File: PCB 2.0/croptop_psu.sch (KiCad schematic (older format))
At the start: 35 parts, among them J3 5V USB, U2 REG71055, U3 FAN5333BSX, U4 MIC23050, U5 TC1014

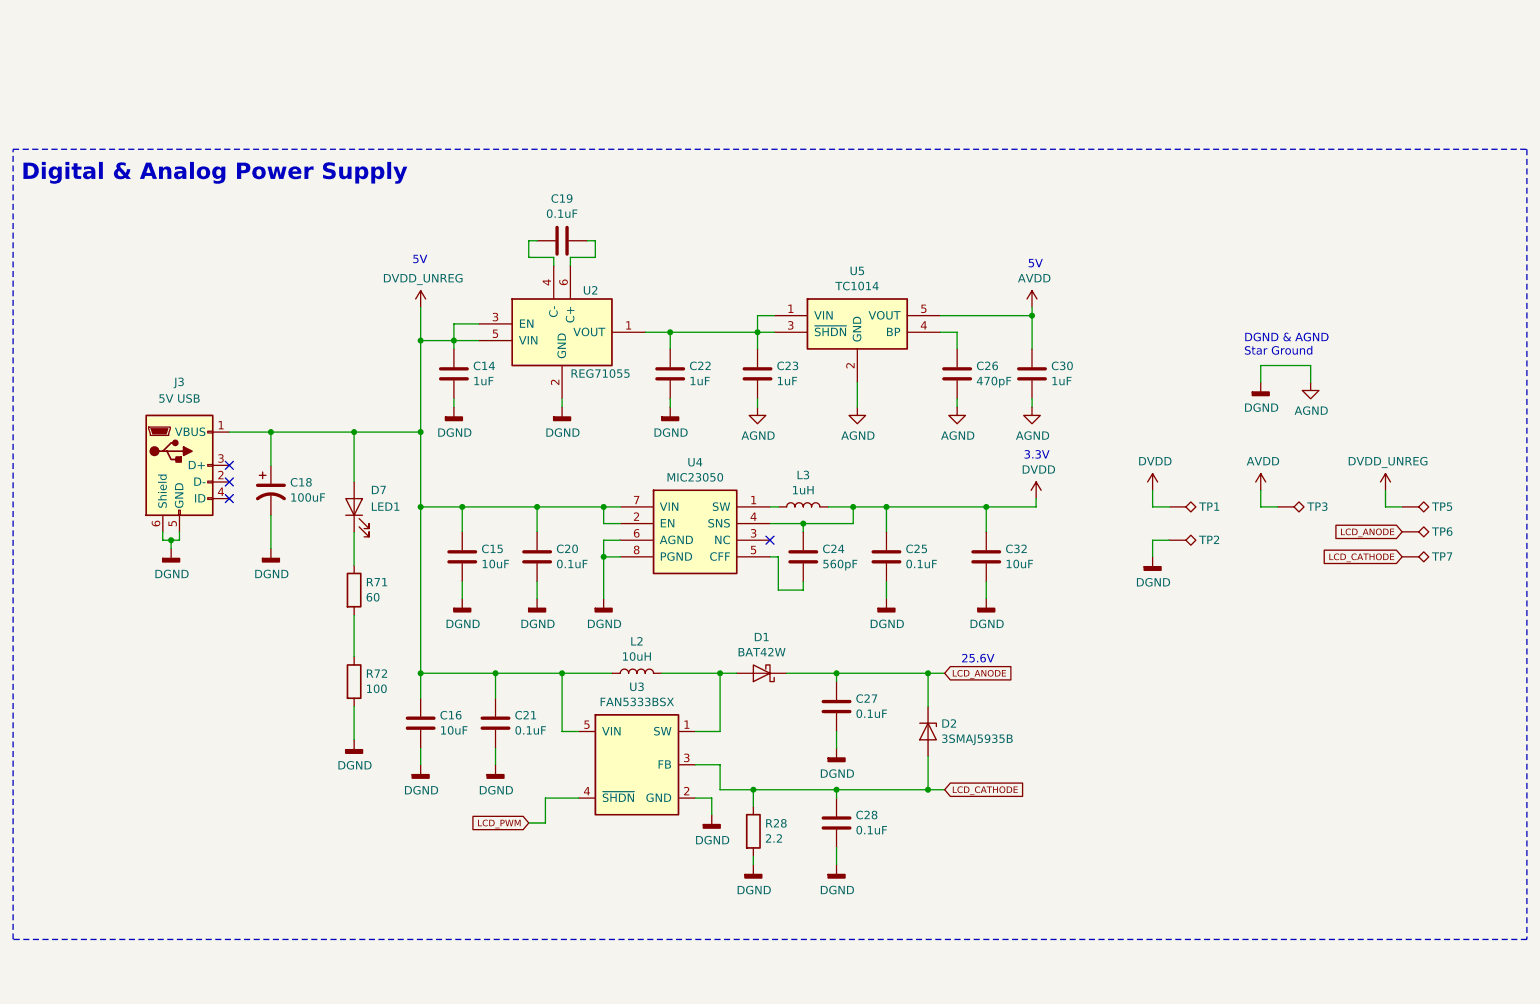
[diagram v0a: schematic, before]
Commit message: Fixed it
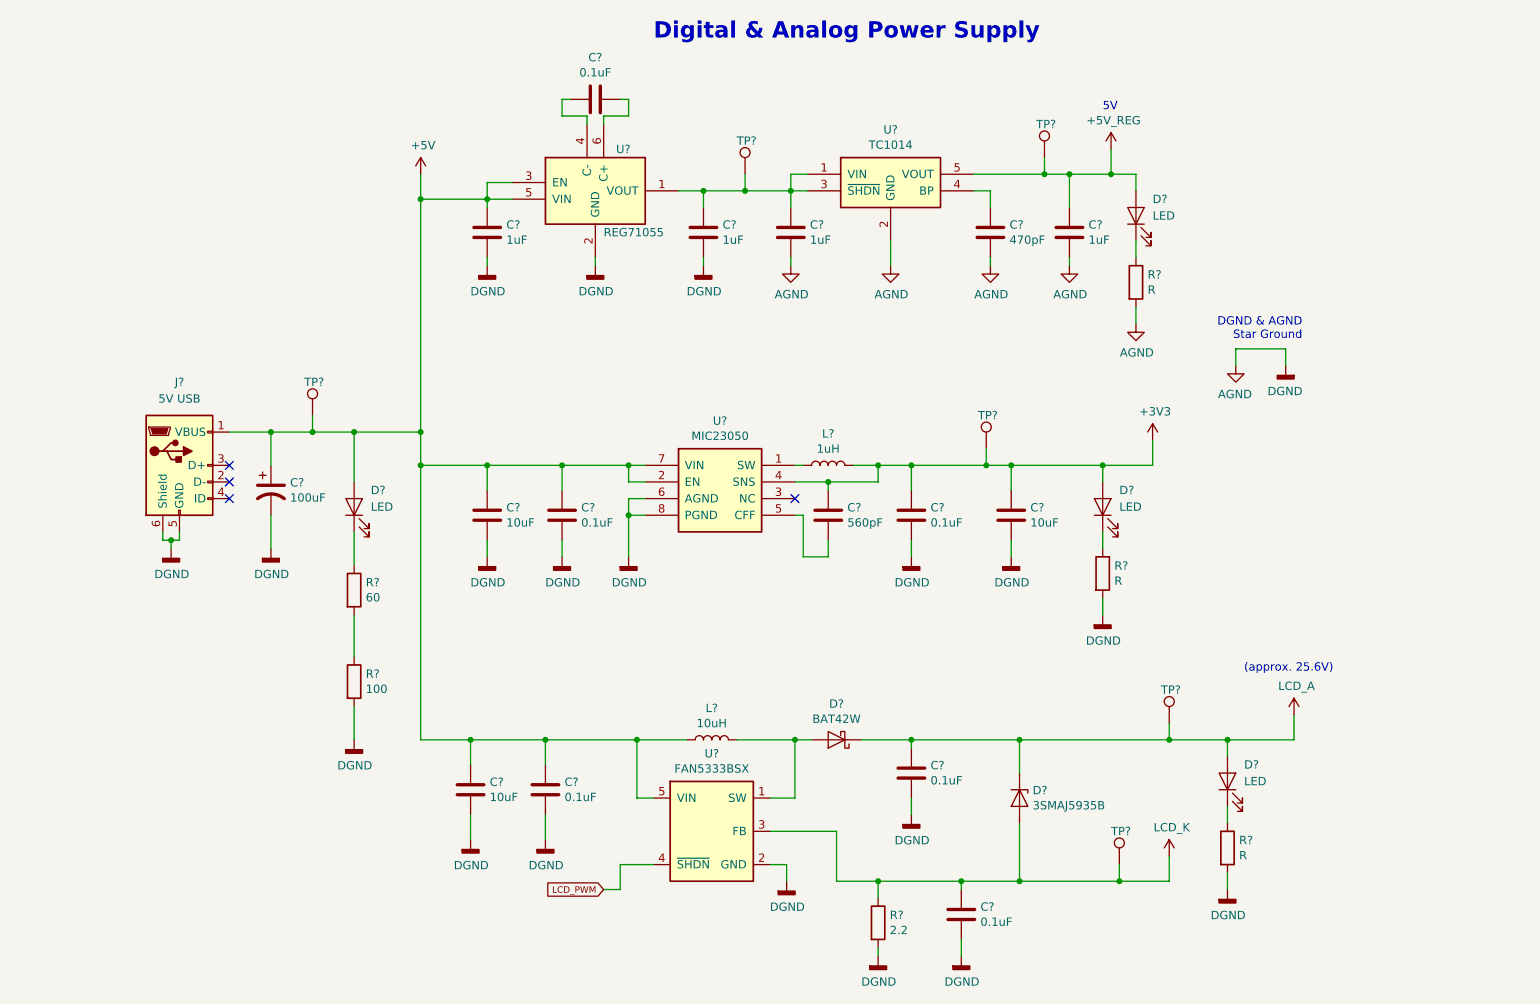
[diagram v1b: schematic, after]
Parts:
- removed TP1, TP2, TP3, TP5, TP6, TP7: TestPoint_Alt, croptop:TestPoint, symbol Connector:TestPoint_Alt
- added D? (x3): LED, LED_SMD:LED_0805_2012Metric, symbol Device:LED
- added R? (x3): R, symbol Device:R
- added TP? (x6): TestPoint, symbol Connector:TestPoint
- D?: renamed from D7; value LED1 -> LED
- renumbered C15 to C?, C20 to C?, C32 to C?, C25 to C?, C16 to C?, C21 to C?, C28 to C?, C27 to C?, C18 to C?, C14 to C?, C22 to C?, C23 to C?, C30 to C?, C19 to C?, C26 to C?, C24 to C?, D2 to D?, D1 to D?, J3 to J?, L3 to L?, L2 to L?, R72 to R?, R71 to R?, R28 to R?, U3 to U?, U4 to U?, U2 to U?, U5 to U?
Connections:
- net AGND: now also R?.2, R?.2, R?.2
- net at C?.1, C?.1, U?.1 (VIN)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: now also TP?.1
- net AVDD renamed +5V_REG
- net +5V_REG: now also D?.2 (A), TP?.1
- net DVDD renamed +3V3
- net +3V3: now also D?.2 (A), TP?.1
- net DVDD_UNREG renamed +5V
- net +5V: now also TP?.1
- net LCD_ANODE renamed LCD_A
- net LCD_A: now also D?.2 (A), TP?.1
- net LCD_CATHODE renamed LCD_K
- net LCD_K: now also TP?.1
- new net: D?.1 (K), R?.1 (x3)
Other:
- note added: "(approx. 25.6V)"
- note removed: "25.6V"
- note removed: "3.3V"
- moved on the sheet: C?, D?, L?, R?, U?
